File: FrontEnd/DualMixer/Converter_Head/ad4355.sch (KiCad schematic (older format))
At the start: 70 parts, among them J401 uFL, J402 uFL, K401 TCM1-83X-1+, K402 TCM1-83X-1+, U401 ADM7170ACPZ-5.0, U402 ADM7170ACPZ-3.3, U403 ADM7170ACPZ-3.3, U404 ADF4355

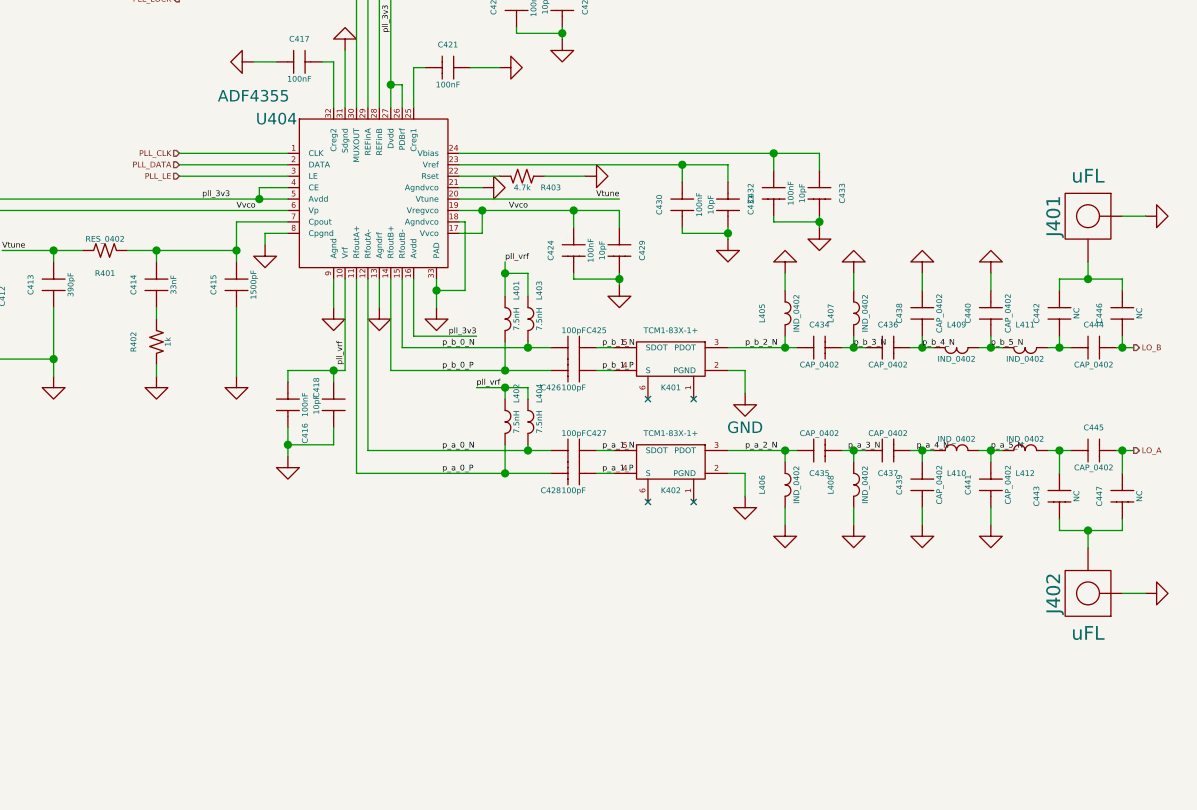
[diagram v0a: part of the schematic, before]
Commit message: sent in production
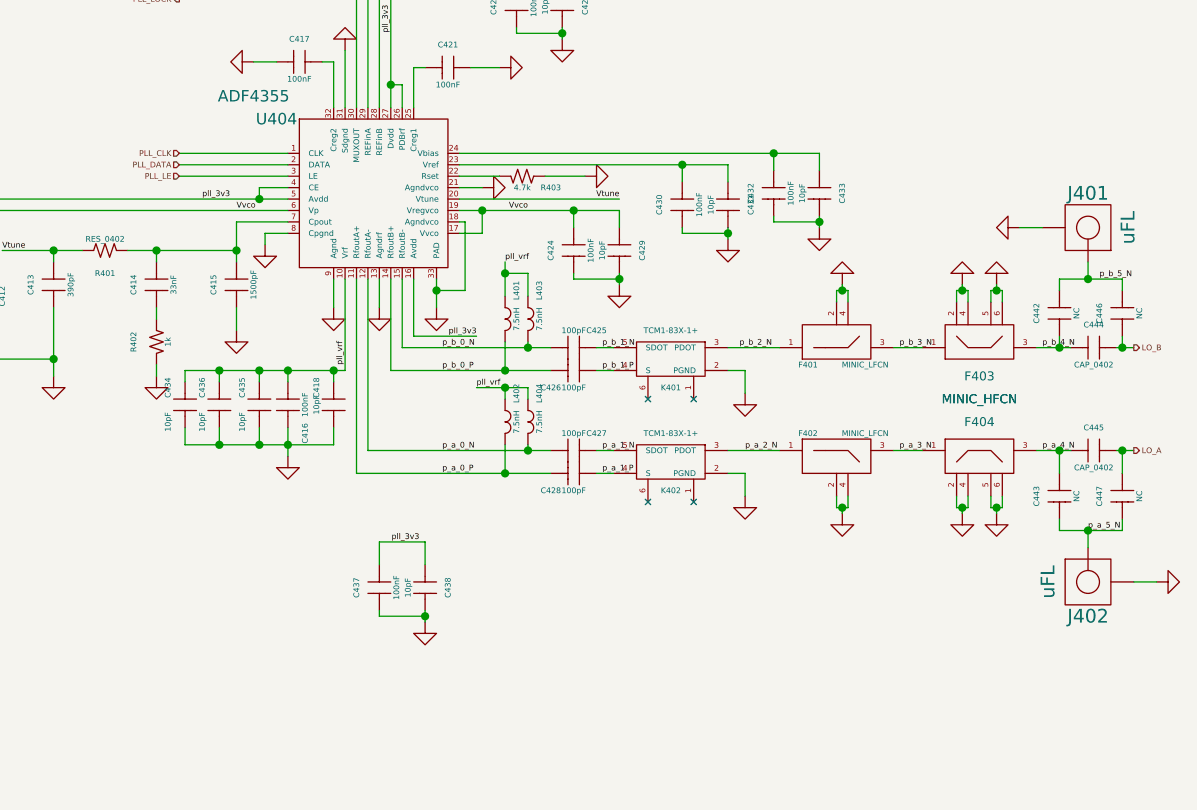
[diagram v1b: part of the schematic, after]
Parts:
- removed C437, C439, C440, C441: CAP_0402, SM0402, symbol passives:CAP_0402
- removed L405, L406, L407, L408, L409, L410, L411, L412: IND_0402, SM0402, symbol passives:IND_0402
- added C437: 100nF, SM0402, symbol passives:CAP_0603
- added F401, F402: MINIC_LFCN, MiniCircuits:FV1206, symbol minic_lfcn:MINIC_LFCN
- added F403, F404: MINIC_HFCN, MiniCircuits:FV1206, symbol minic_hfcn:MINIC_HFCN
- C434, C435, C436, C438: value CAP_0402 -> 10pF
- J401, J402: footprint (none) -> Connectors_RF:U.FL-R-SMT-1
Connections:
- net GND: now also C434.2, C435.2, C436.2, J401.2 (GND), J402.2 (GND), C437.2, F401.2 (GND), F401.4 (GND), F402.2 (GND), F402.4 (GND), F403.2 (GND), F403.4 (GND), F403.5 (GND), F403.6 (GND), F404.2 (GND), F404.4 (GND), F404.5 (GND), F404.6 (GND); no longer J401.1 (RF), J402.1 (RF)
- net p_a_2_N: now also F402.1 (RFIN); no longer C435.1
- net p_a_3_N: now also F402.3 (RFOUT), F404.1 (RFIN); no longer C435.2
- net p_a_4_N: now also C443.1, C445.1, F404.3 (RFOUT)
- net p_a_5_N: now also C443.2, C447.2, J402.1 (RF)
- net p_b_2_N: now also F401.1 (RFIN); no longer C434.1
- net p_b_3_N: now also F401.3 (RFOUT), F403.1 (RFIN); no longer C434.2, C436.1
- net p_b_4_N: now also C442.1, C444.1, F403.3 (RFOUT); no longer C436.2, C438.1
- net p_b_5_N: now also C442.2, C446.2, J401.1 (RF)
- net pll_3v3: now also C438.1, C437.1
- net pll_vrf: now also C434.1, C435.1, C436.1
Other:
- moved on the sheet: J401, J402
